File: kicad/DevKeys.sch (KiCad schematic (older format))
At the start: 12 parts, among them SW1 SWITCH_PUSH, SW10 SWITCH_PUSH, SW2 SWITCH_PUSH, SW3 SWITCH_PUSH, SW4 SWITCH_PUSH, SW5 SWITCH_PUSH, SW6 SWITCH_PUSH, SW7 SWITCH_PUSH, SW8 SWITCH_PUSH, SW9 SWITCH_PUSH, U1 ARDUINO_MICRO_SHIELD

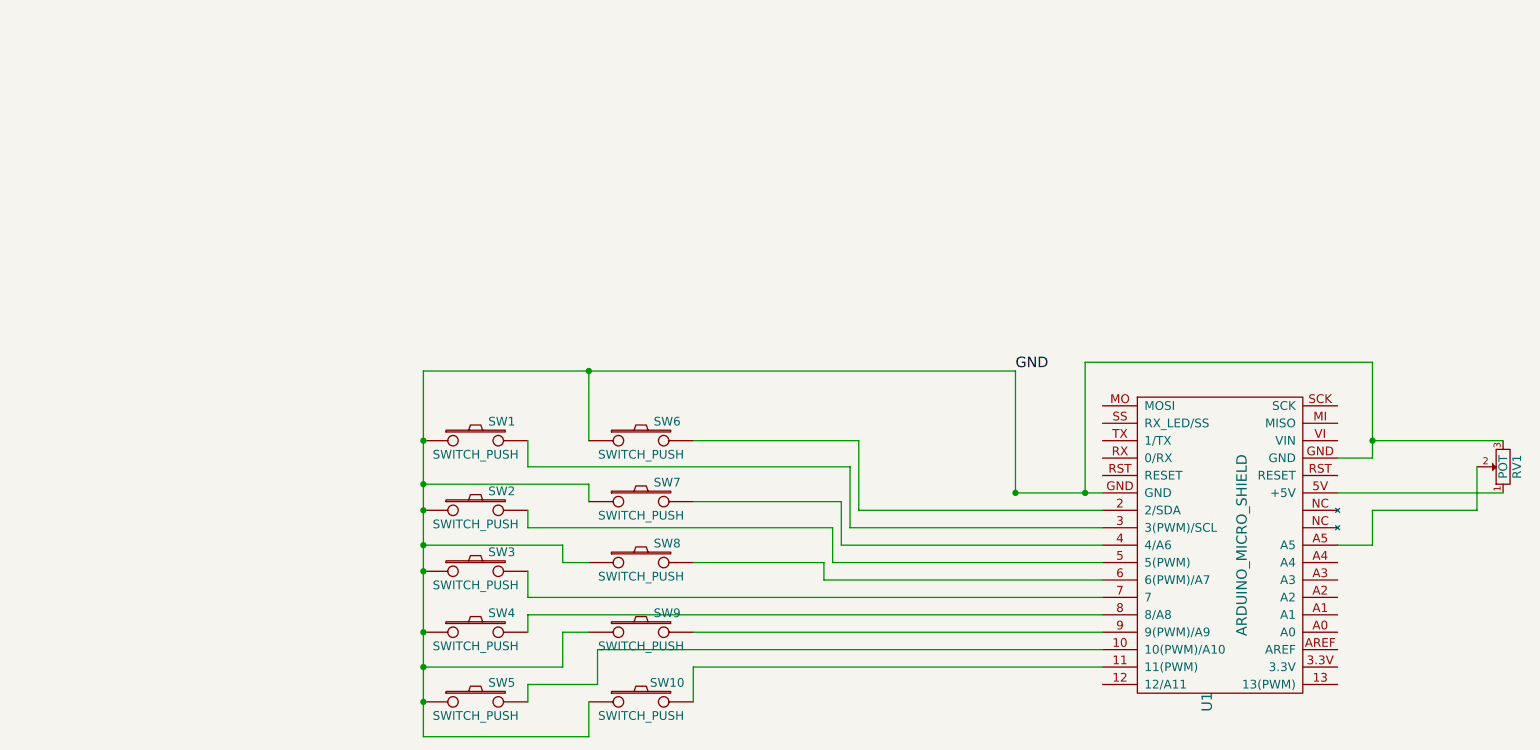
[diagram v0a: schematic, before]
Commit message: neues Platinen-Layout
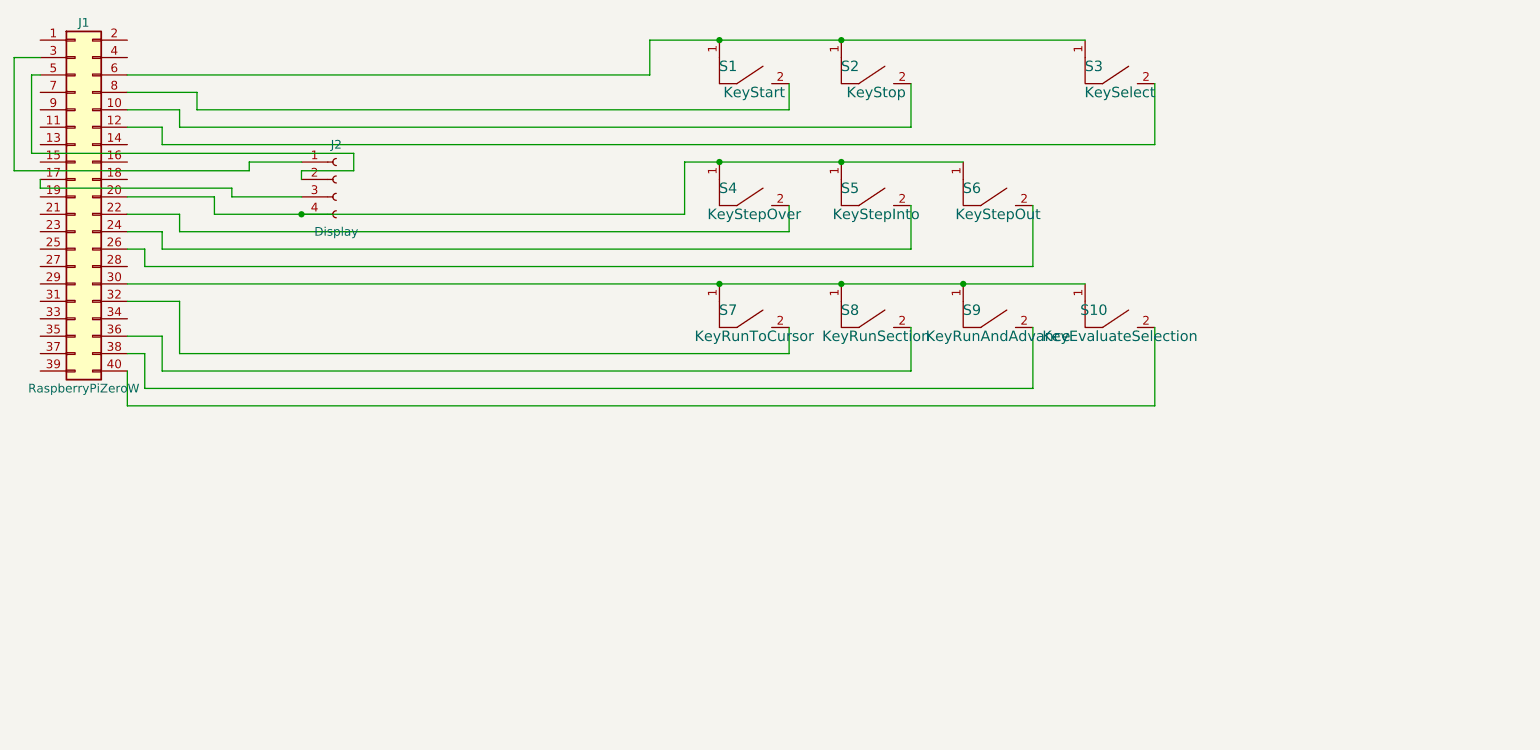
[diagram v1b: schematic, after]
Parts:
- removed RV1: POT, Potentiometers:Potentiometer_WirePads, symbol POT-RESCUE-DevKeys
- removed SW1, SW10, SW2, SW3, SW4, SW5, SW6, SW7, SW8, SW9: SWITCH_PUSH, footprints:CHERRY_PCB_100H, symbol SWITCH_PUSH
- removed U1: ARDUINO_MICRO_SHIELD, arduino_micro_shield:ARDUINO_MICRO_SHIELD, symbol ARDUINO_MICRO_SHIELD
- added J1: RaspberryPiZeroW, Pin_Headers:Pin_Header_Straight_2x20_Pitch2.54mm, symbol Conn_02x20_Odd_Even
- added J2: Display, Socket_Strips:Socket_Strip_Straight_1x04_Pitch2.54mm, symbol Conn_01x04_Female
- added S1: KeyStart, mx1a:MX1A, symbol MX1A
- added S10: KeyEvaluateSelection, mx1a:MX1A, symbol MX1A
- added S2: KeyStop, mx1a:MX1A, symbol MX1A
- added S3: KeySelect, mx1a:MX1A, symbol MX1A
- added S4: KeyStepOver, mx1a:MX1A, symbol MX1A
- added S5: KeyStepInto, mx1a:MX1A, symbol MX1A
- added S6: KeyStepOut, mx1a:MX1A, symbol MX1A
- added S7: KeyRunToCursor, mx1a:MX1A, symbol MX1A
- added S8: KeyRunSection, mx1a:MX1A, symbol MX1A
- added S9: KeyRunAndAdvance, mx1a:MX1A, symbol MX1A
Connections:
- new net: J1.10 (Pin_10), S2.2
- new net: J1.12 (Pin_12), S3.2
- new net: J1.17 (Pin_17), J2.3 (Pin_3)
- new net: J1.20 (Pin_20), J2.4 (Pin_4), S4.1, S5.1, S6.1
- new net: J1.22 (Pin_22), S4.2
- new net: J1.24 (Pin_24), S5.2
- new net: J1.26 (Pin_26), S6.2
- new net: J1.3 (Pin_3), J2.1 (Pin_1)
- new net: J1.30 (Pin_30), S10.1, S7.1, S8.1, S9.1
- new net: J1.32 (Pin_32), S7.2
- new net: J1.36 (Pin_36), S8.2
- new net: J1.38 (Pin_38), S9.2
- new net: J1.40 (Pin_40), S10.2
- new net: J1.5 (Pin_5), J2.2 (Pin_2)
- new net: J1.6 (Pin_6), S1.1, S2.1, S3.1
- new net: J1.8 (Pin_8), S1.2
